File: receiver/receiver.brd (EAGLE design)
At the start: 100 x 80 mm, 4 parts, among them Q1 3.3

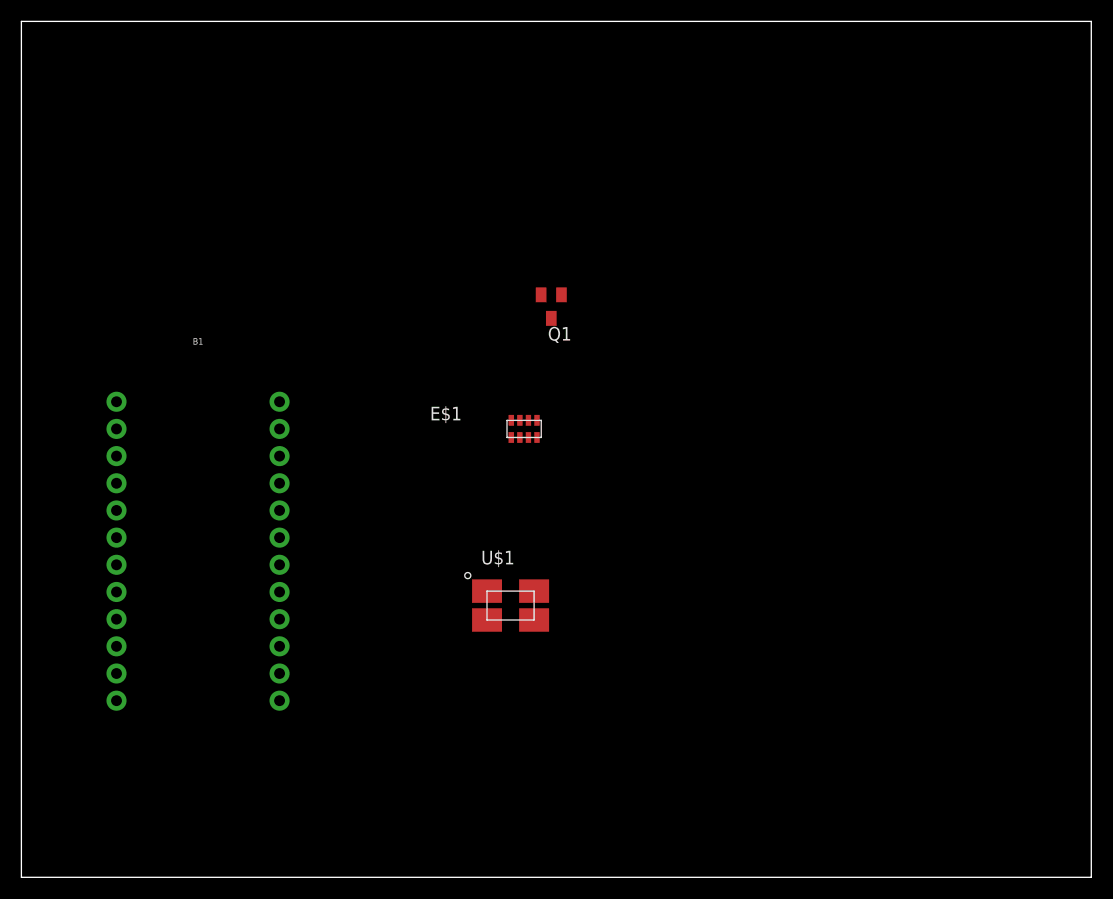
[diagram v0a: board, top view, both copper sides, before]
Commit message: layout components
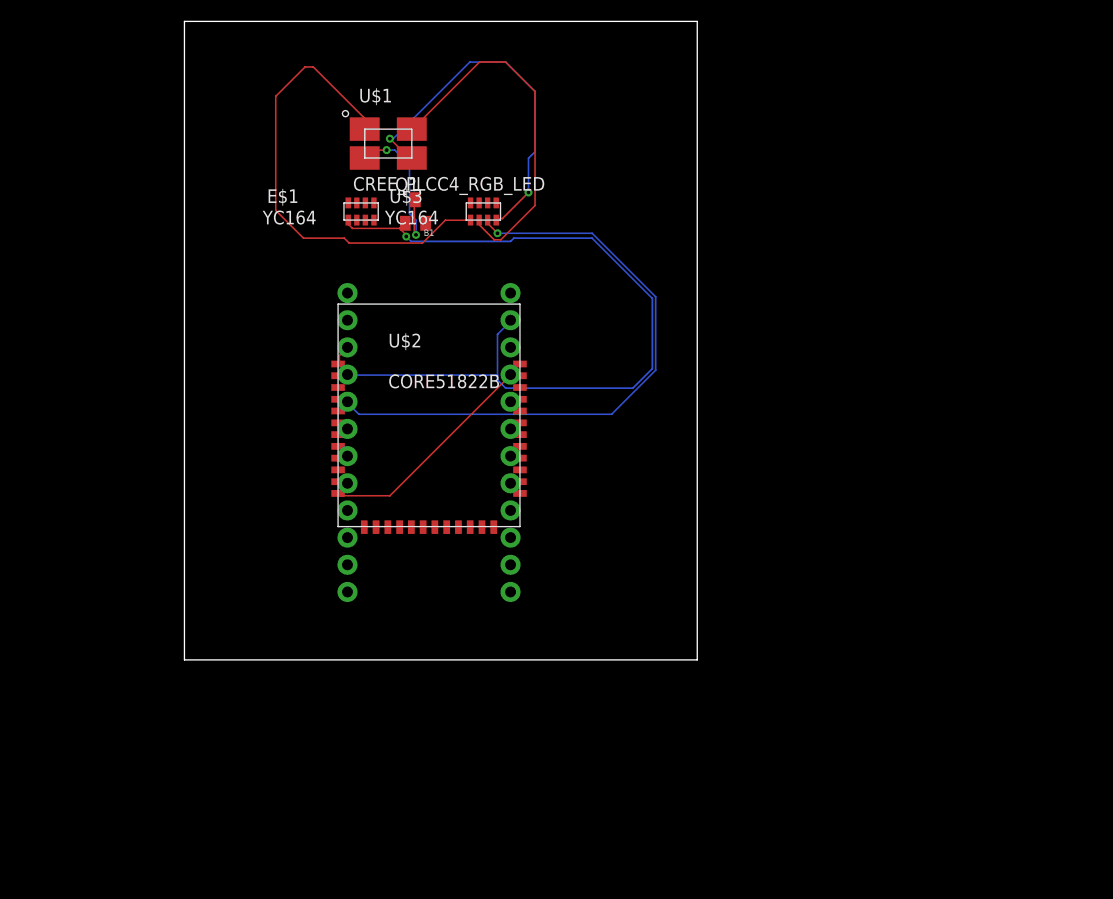
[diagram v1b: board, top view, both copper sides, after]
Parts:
- added U$2: CORE51822B, core51822b:CORE51822B
- added U$3: YC164, yc164:YC164
- E$1: value (none) -> YC164
- U$1: value (none) -> CREE_PLCC4_RGB_LED
- moved U$1 44.7 mm to (34.3, 68.6)
- moved E$1 25.4 mm to (31.8, 62.2)
- moved B1 23.9 mm to (38.1, 41.9)
- moved Q1 15.5 mm to (36.8, 62.2), turned to 0 degrees
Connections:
- removed net RAW: B1.24
- new net N$1: B1.24, Q1.3, U$1.P$2
- new net N$10: U$1.P$4, U$3.P$6
- new net N$11: U$1.P$1, U$3.P$5
- new net N$12: U$3.P$2, U$3.P$3
- new net N$14: U$1.P$3, U$3.P$8
- new net N$2: B1.22
- new net N$3: B1.20, U$3.P$4
- new net N$4: B1.19, U$3.P$1
- new net N$5: B1.5, U$3.P$7
- new net N$6: B1.6
- new net N$7: B1.1, E$1.P$7, E$1.P$8
- new net N$8: E$1.P$1, E$1.P$2, E$1.P$3, E$1.P$4, U$2.P25
- net GND: now also E$1.P$5, Q1.1, U$2.GND0, U$2.GND1
- net VCC: now also Q1.2, U$2.VCC
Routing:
- net GND: track 0.00 -> 78.5 mm, vias 0 -> 1
- net N$5: track 0.00 -> 56.8 mm, vias 0 -> 1
- net N$11: track 0.00 -> 43.5 mm
- net N$14: track 0.00 -> 34.3 mm, vias 0 -> 2
- net N$10: track 0.00 -> 33.5 mm
- net VCC: track 0.00 -> 20.9 mm
- net N$1: track 0.00 -> 15.3 mm, vias 0 -> 2
- net N$7: track 0.00 -> 0.81 mm
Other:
- board size 100 x 80 mm -> 47.9 x 59.7 mm
